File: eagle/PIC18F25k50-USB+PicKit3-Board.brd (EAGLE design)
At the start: 18 parts, among them J1 PIC-ICSP-PK3, J2 USB-PRINT, J3 RA[0..4], J4 RC[0..3], J5 PWR+SCI+USB, J6 RB[0..7], SW1 PB-1P-1T

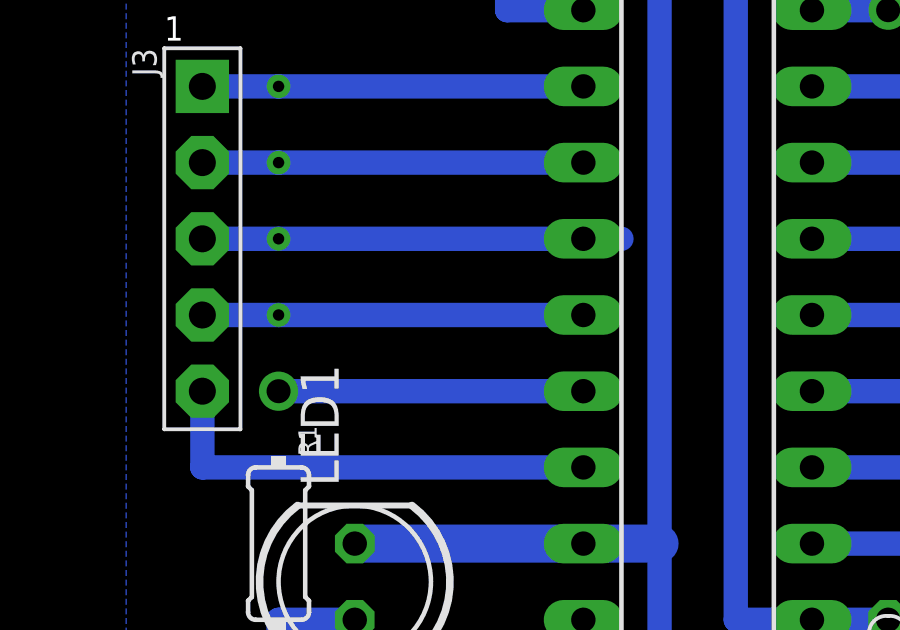
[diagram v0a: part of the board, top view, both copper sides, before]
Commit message: ...
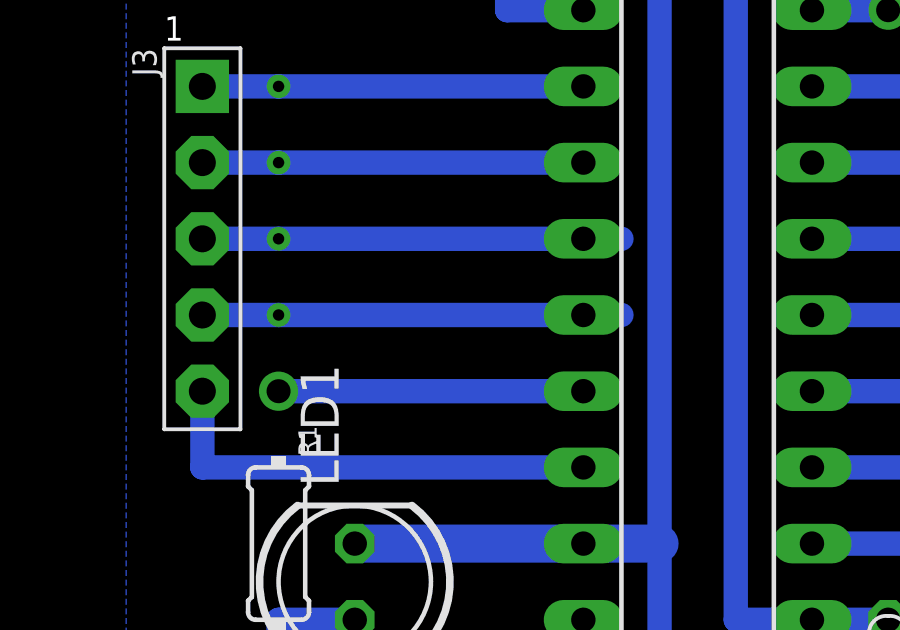
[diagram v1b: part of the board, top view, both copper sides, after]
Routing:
- net A3: track 13.3 -> 14.0 mm

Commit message: ...
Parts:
- C5: value 100uF -> 100μF
- R1, R5: value 330 -> 330Ω
- R2, R3: value 100 -> 100Ω
- R4: value 10k -> 10kΩ
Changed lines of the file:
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@@
         <element name="C2" library="c" package="C025-015X024" value="100n" x="25.4" y="31.75" />
         <element name="J2" library="usb" package="USB-B-PRINT" value="USB-PRINT" x="17.78" y="7.62" rot="R90" />
-        <element name="R1" library="r" package="0204/10" value="330" x="5.08" y="35.56" rot="R270" />
+        <element name="R1" library="r" package="0204/10" value="330Ω" x="5.08" y="35.56" rot="R270" />
         <element name="LED1" library="led" package="LED5MM" value="" x="7.62" y="34.29" rot="R90" />
-        <element name="C5" library="c" package="E2,5-5" value="100uF" x="30.48" y="11.43" rot="R90" />
+        <element name="C5" library="c" package="E2,5-5" value="100μF" x="30.48" y="11.43" rot="R90" />
         <element name="J4" library="pinconn" package="CONN-4P" value="RC[0..3]" x="2.54" y="24.13" rot="R270" />
         <element name="J5" library="pinconn" package="CONN-6P" value="PWR+SCI+USB" x="35.56" y="26.67" rot="R90" />
         <element name="J6" library="pinconn" package="CONN-8P" value="RB[0..7]" x="35.56" y="35.56" rot="R90" />
         <element name="J3" library="pinconn" package="CONN-5P-N" value="RA[0..4]" x="2.54" y="45.72" rot="R270" />
-        <element name="R2" library="r" package="0204/7-V" value="100" x="25.4" y="57.15" />
-        <element name="R3" library="r" package="0204/7-V" value="100" x="27.94" y="54.61" />
+        <element name="R2" library="r" package="0204/7-V" value="100Ω" x="25.4" y="57.15" />
+        <element name="R3" library="r" package="0204/7-V" value="100Ω" x="27.94" y="54.61" />
         <element name="U$1" library="mcu" package="PIC18F2550-V" value="PIC18F2550-I/SPLABEL" x="19.05" y="38.1" />
-        <element name="R4" library="r" package="0204/10" value="10k" x="15.24" y="55.88" />
+        <element name="R4" library="r" package="0204/10" value="10kΩ" x="15.24" y="55.88" />
         <element name="SW1" library="sw" package="PB-1P1T" value="PB-1P-1T" x="10.16" y="63.5" />
-        <element name="R5" library="r" package="0204/10" value="330" x="15.24" y="58.42" rot="R180" />
+        <element name="R5" library="r" package="0204/10" value="330Ω" x="15.24" y="58.42" rot="R180" />
         <element name="LED2" library="led" package="LED5MM" value="" x="3.81" y="58.42" rot="R180" />
       </elements>
